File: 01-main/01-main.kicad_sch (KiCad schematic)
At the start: 96 parts, among them J1 USB_C_Receptacle_USB2.0, J10 front, J11 ToF_R, J12 ToF_RB, J13 ToF_L, J14 ToF_LB, J15 PWR_board_GND, J16 PWR_board_GND, J17 PWR_board_VIN, J18 PWR_board_VOUT, J19 XT60_LiPo, J2 Motor_RF, J20 UI_conn, J21 LOADCELL_R, J22 LOADCELL_L, J23 Conn_01x08, J3 Motor_RB, J4 Motor_LF, J5 Motor_LB, J6 OpenMV, J7 Conn_01x10, J8 Top, J9 Conn_01x10, SW1 SW_RST, SW2 SW_BOOT0, U1 STM32H723ZETx, U10 REG 6V, U11 NJU77551F, U12 NJU77551F, U2 CH340E, U4 REG 3V3, U6 REG 5V, U7 REG 6V, U8 REG 6V, U9 REG 6V, Y1 32.768kHz, Y2 24MHz

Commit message: がんばる
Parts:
- removed C10: 4.7uF, symbol Device:C
- removed C11, C12, C13, C14, C16, C20, C21, C4, C5, C6, C7, C8: 100nF, symbol Device:C
- removed C15, C19, C9: 1uF, symbol Device:C
- removed C17, C18: 2.2uF, symbol Device:C
- removed C22, C23: 1.5pF, symbol Device:C
- removed C24, C25: 33pF, symbol Device:C
- removed C26, C27, C33, C35, C37, C39: 0.1u, symbol Device:C
- removed C28, C30: 10u, symbol Device:C
- removed C29, C31: 22u, symbol Device:C
- removed C32, C34, C36, C38: 0.33u, symbol Device:C
- removed D1, D2: LED, symbol Device:LED
- removed FB1: FerriteBead, symbol Device:FerriteBead
- removed J1: USB_C_Receptacle_USB2.0, symbol Connector:USB_C_Receptacle_USB2.0
- removed J10: front, symbol Connector_Generic:Conn_01x10
- removed J11: ToF_R, symbol Connector_Generic:Conn_01x04
- removed J12: ToF_RB, symbol Connector_Generic:Conn_01x04
- removed J13: ToF_L, symbol Connector_Generic:Conn_01x04
- removed J14: ToF_LB, symbol Connector_Generic:Conn_01x04
- removed J15, J16: PWR_board_GND, symbol Connector_Generic:Conn_01x01
- removed J17: PWR_board_VIN, symbol Connector_Generic:Conn_01x01
- removed J18: PWR_board_VOUT, symbol Connector_Generic:Conn_01x01
- removed J19: XT60_LiPo, symbol Connector_Generic:Conn_01x02
- removed J2: Motor_RF, symbol Connector_Generic:Conn_01x03
- removed J20: UI_conn, symbol Connector_Generic:Conn_01x04
- removed J21: LOADCELL_R, symbol Connector_Generic:Conn_01x04
- removed J22: LOADCELL_L, symbol Connector_Generic:Conn_01x04
- removed J23: Conn_01x08, symbol Connector_Generic:Conn_01x08
- removed J3: Motor_RB, symbol Connector_Generic:Conn_01x03
- removed J6: OpenMV, symbol Connector_Generic:Conn_01x04
- removed J7, J9: Conn_01x10, symbol Connector_Generic:Conn_01x10
- removed J8: Top, symbol Connector_Generic:Conn_02x03_Counter_Clockwise
- removed R6: 330k, symbol Device:R
- removed R7, R8: 330, symbol Device:R
- removed SW1: SW_RST, symbol Switch:SW_Push
- removed SW2: SW_BOOT0, symbol Switch:SW_SPDT
- removed U1: STM32H723ZETx, Package_QFP:LQFP-144_20x20mm_P0.5mm, symbol MCU_ST_STM32H7:STM32H723ZETx
- removed U10, U7, U8, U9: REG 6V, Package_TO_SOT_SMD:TO-252-2, symbol Regulator_Linear:LF50_TO252
- removed U11, U12: NJU77551F, Package_TO_SOT_SMD:SOT-23-5, symbol Amplifier_Operational:OPA196xDBV
- removed U13: ~, symbol S11059:S11059
- removed U2: CH340E, Package_SO:MSOP-10_3x3mm_P0.5mm, symbol Interface_USB:CH340E
- removed U3: ~, symbol MPU6050:MPU6050
- removed U4: REG 3V3, Package_TO_SOT_SMD:TO-252-2, symbol Regulator_Linear:LF33_TO252
- removed U5: ~, symbol BNO055:AE-BNO055-BO
- removed U6: REG 5V, Package_TO_SOT_SMD:TO-252-2, symbol Regulator_Linear:LF50_TO252
- removed Y1: 32.768kHz, symbol Device:Crystal
- removed Y2: 24MHz, symbol Device:Crystal
- added J2: WRITER CONN, Connector_PinHeader_2.54mm:PinHeader_2x04_P2.54mm_Vertical, symbol Connector_Generic:Conn_02x04_Counter_Clockwise
- added J2: LOADCELL_R, symbol Connector_Generic:Conn_01x04
- added J3: LOADCELL_L, symbol Connector_Generic:Conn_01x04
- added J6, J7: Motor_R1, symbol Connector_Generic:Conn_01x03
- added J8: ToLINE, symbol Connector_Generic:Conn_01x04
- added Q1: 2SA1015, Package_TO_SOT_THT:TO-92_Inline, symbol Transistor_BJT:2SA1015
- added R14, R15, R16: 330k, symbol Device:R
- added U2: STM32F446RETx, Package_QFP:LQFP-64_10x10mm_P0.5mm, symbol MCU_ST_STM32F4:STM32F446RETx
- added U2: MAX485E, symbol Interface_UART:MAX485E
- added U3: ~, symbol BNO055:AE-BNO055-BO
- added U5, U6: NJU77551F, Package_TO_SOT_SMD:SOT-23-5, symbol Amplifier_Operational:OPA196xDBV
- C1: value 100nF -> 0.1u
- C2: value 100nF -> 100n
- C3: value 100nF -> 4.7u
- J4: value Motor_LF -> Motor_R1
- J5: value Motor_LB -> Motor_R1
- R1: value 10K -> 220
- R12, R9: value 330k -> 330
- R2: value 5.1k -> 7.5k
- R3: value 5.1k -> 2.2k
- R4: value R -> 2.2k
- R5: value R -> 10k; footprint (none) -> Resistor_SMD:R_0805_2012Metric; LCSC (none) -> C17414
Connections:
- net MotorLB is gone; now on net GND: J5.3 (Pin_3)
- net MotorLF is gone; now on net GND: J4.3 (Pin_3)
- net +3V3: now also J2.4 (Pin_4), J2.8 (Pin_8), J3.4 (Pin_4), U2.1 (VBAT), U2.13 (VDDA), U2.19 (VDD), U2.32 (VDD), U2.48 (VDD), U2.64 (VDD), U3.1 (VIN), U5.5 (V+), U6.5 (V+); no longer C1.1, C2.1, C3.1
- net +5V: now also C1.1, R3.1, Q1.2 (C), U2.8 (VCC)
- net BOOT0: now also R5.1, J2.5 (Pin_5), U2.60 (BOOT0); no longer R1.2
- net GND: now also C2.1, R1.2, R4.1, R5.2, J2.1 (Pin_1), J2.6 (Pin_6), J3.1 (Pin_1), J6.3 (Pin_3), J7.3 (Pin_3), R15.2, U2.12 (VSSA), U2.18 (VSS), U2.31 (VSS), U2.47 (VSS), U2.5 (GND), U2.63 (VSS), U3.2 (GND), U5.2 (V-), U6.2 (V-); no longer C2.2, J4.2 (Pin_2), J5.2 (Pin_2), R2.2, R3.2, R4.2
- net I2C1_SCL: now also U2.58 (PB6), U3.4 (SCL)
- net I2C1_SDA: now also U2.59 (PB7), U3.3 (SDA)
- net I2C2_SCL: now also U2.29 (PB10)
- net I2C2_SDA: now also U2.53 (PC12)
- net LOADCEL_L: now also R16.1, U6.1; no longer R12.1
- net LOADCEL_R: now also R14.1, U5.1; no longer R9.1
- net NRST: now also C2.2, J2.3 (Pin_3), U2.7 (NRST)
- net UART1_RX: now also J2.2 (Pin_2), U2.43 (PA10)
- net UART1_TX: now also J2.4 (Pin_4), U2.42 (PA9)
- net at R10.1: now also R14.2, U5.4 (-)
- net at R11.2: now also R15.1, U6.3 (+)
- net at R13.1: now also R9.2, U5.3 (+); no longer R10.2
- net at R11.1: now also J3.2 (Pin_2); no longer R12.2
- net STS_SIG: now reaches J4.1 (Pin_1)
- net STS_SIG: now also J5.1 (Pin_1), J6.1 (Pin_1), J7.1 (Pin_1), U2.6 (A)
- net at R2.1: now also Q1.3 (B)
- net at R1.1: now also Q1.1 (E), U2.2 (~{RE}), U2.3 (DE)
- net Buzzer: no longer names the net of BZ1.1 (-)
- new net: J3.3 (Pin_3), R12.2
- new net: R12.1, R16.2, U6.4 (-)
- new net: J2.2 (Pin_2), R9.1
- new net: J2.3 (Pin_3), R10.2
- new net: C3.1, U2.30 (VCAP_1)
- new net: R3.2, R4.2, U2.7 (B)
- new net: R2.2, U2.4 (DI)
- new net +6V: J4.2 (Pin_2), J5.2 (Pin_2), J6.2 (Pin_2), J7.2 (Pin_2)
- no-connect marks 73 -> 6
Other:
- note removed: "CONN"
- note removed: "LINE SENSOR"
- note removed: "LOADCELL"
- note removed: "MOTOR"
- note removed: "POWER"
- note removed: "SENSOR"
- note removed: "STM32H723ZGT6"

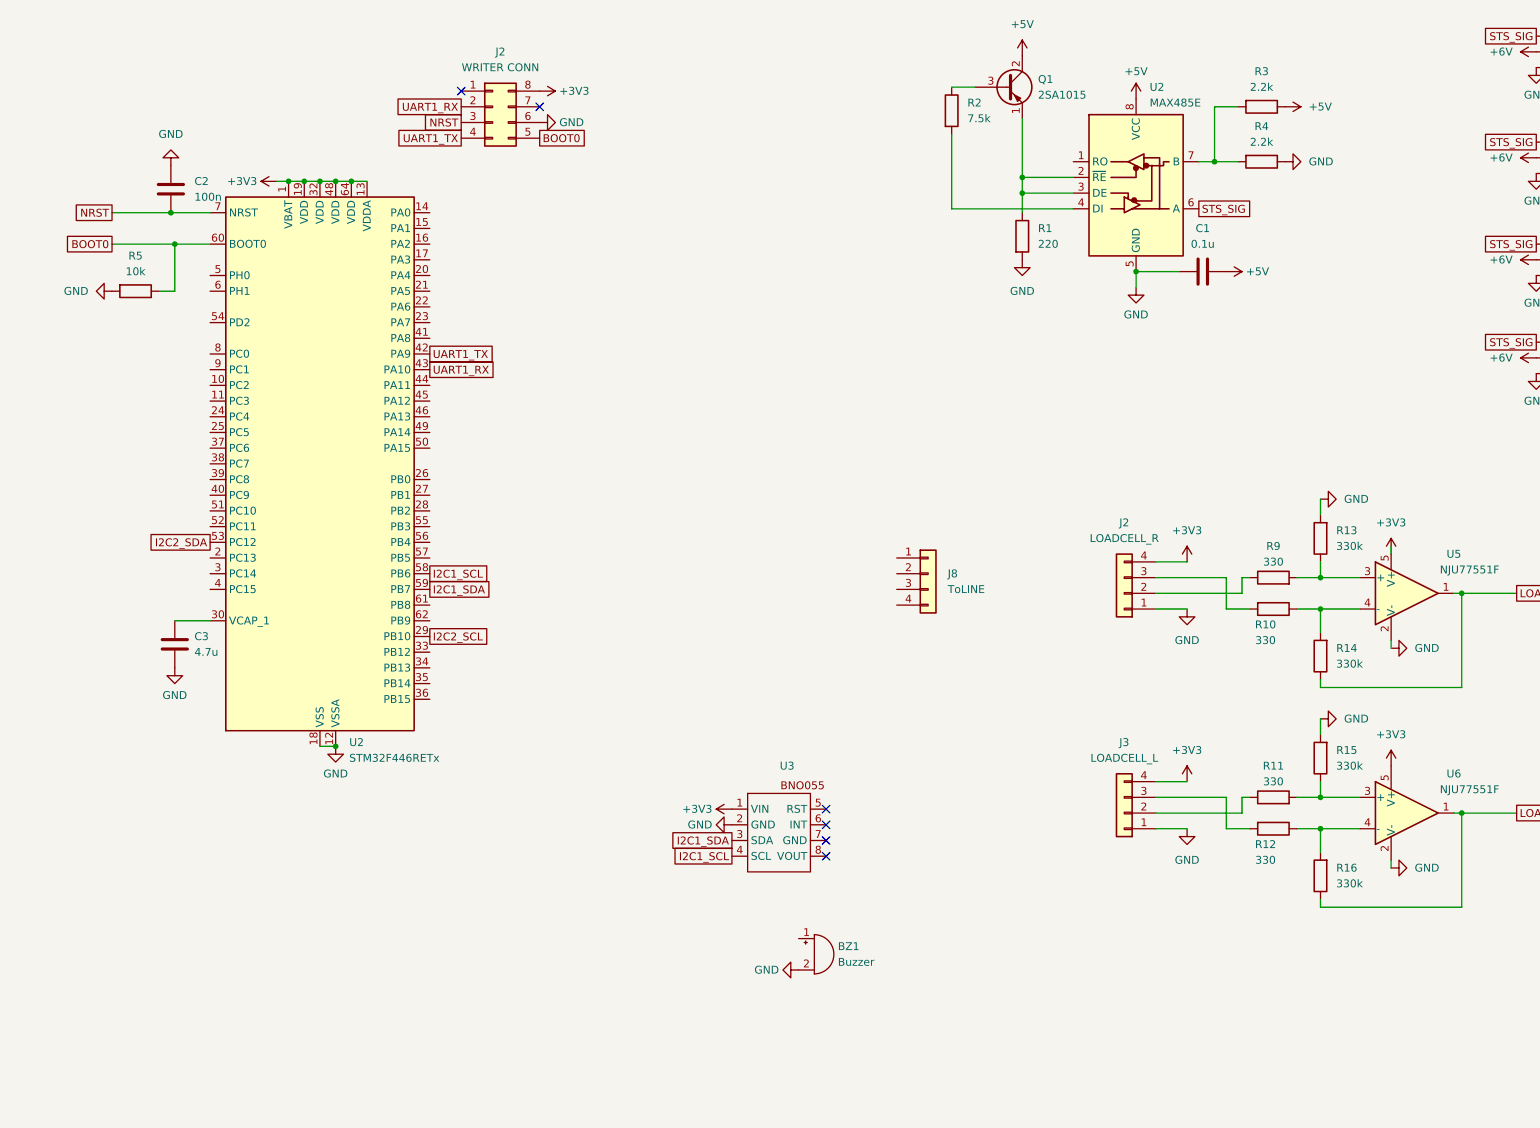
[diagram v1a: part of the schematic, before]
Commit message: いっぱい増えた
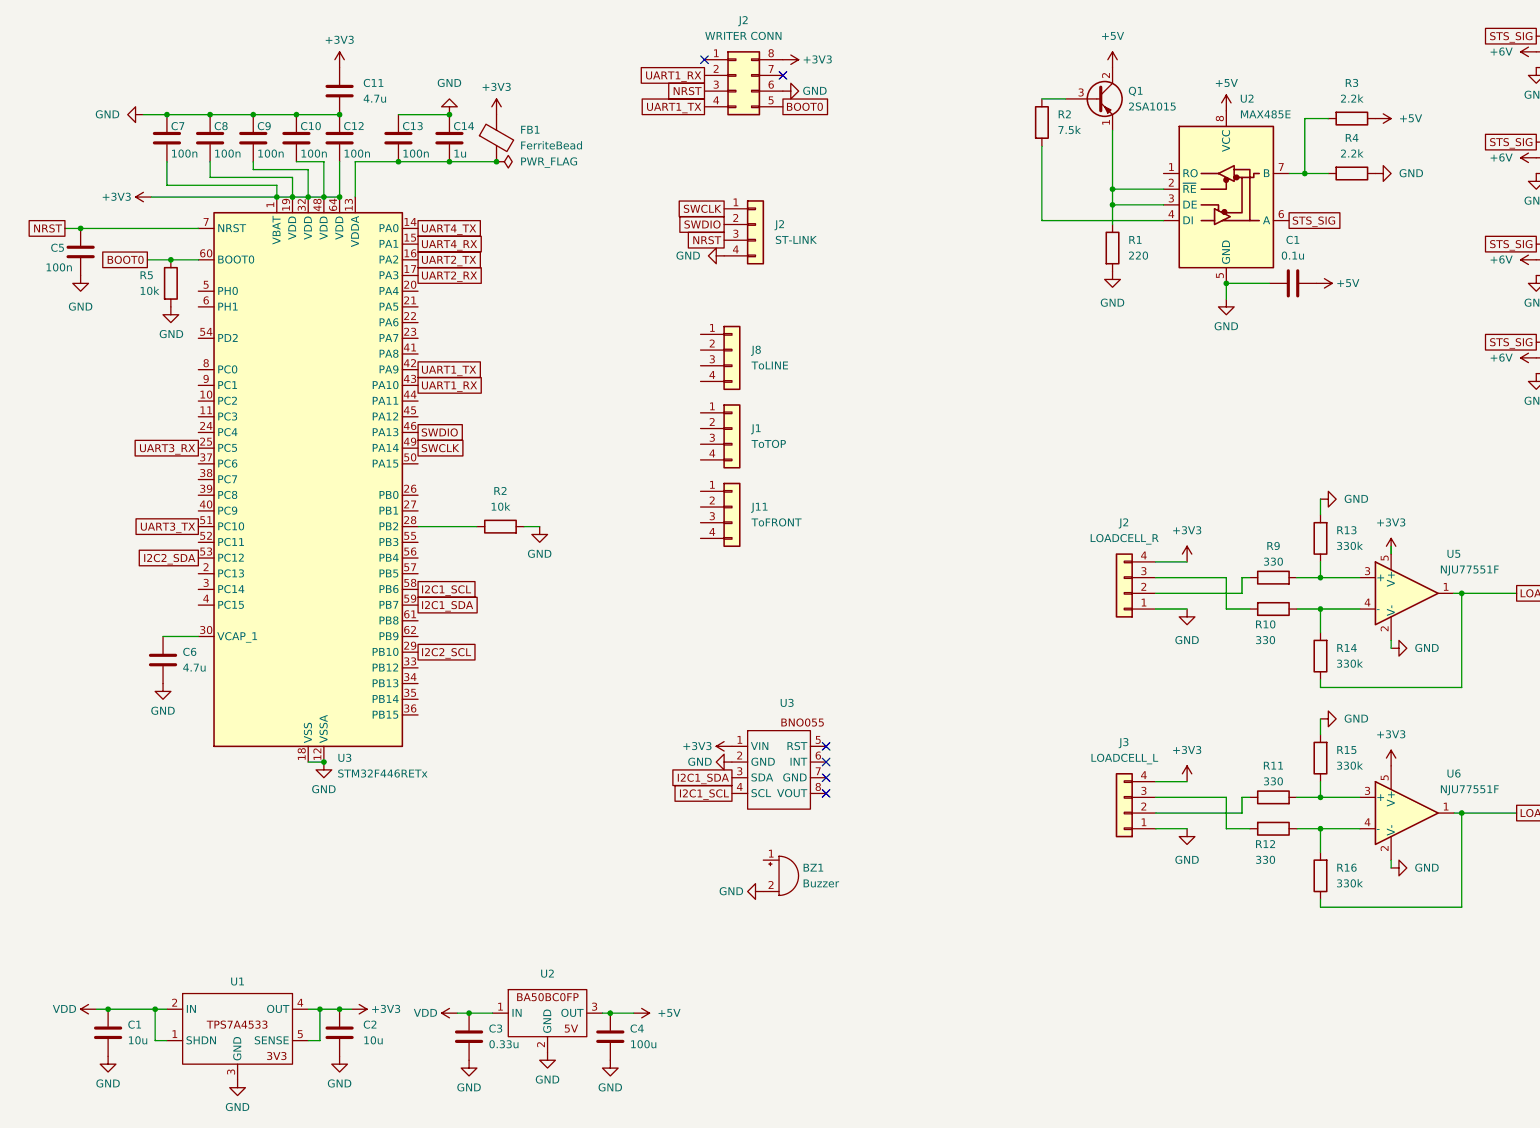
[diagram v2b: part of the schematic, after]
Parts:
- removed U2: STM32F446RETx, Package_QFP:LQFP-64_10x10mm_P0.5mm, symbol MCU_ST_STM32F4:STM32F446RETx
- added C1: 10u, Capacitor_SMD:C_0603_1608Metric, symbol Device:C
- added C10, C12, C13, C5, C7, C8, C9: 100n, Capacitor_SMD:C_0402_1005Metric, symbol Device:C
- added C11, C6: 4.7u, Capacitor_SMD:C_0402_1005Metric, symbol Device:C
- added C14: 1u, Capacitor_SMD:C_0402_1005Metric, symbol Device:C
- added C4: 100u, Capacitor_SMD:C_1206_3216Metric, symbol Device:C
- added FB1: FerriteBead, Resistor_SMD:R_0805_2012Metric, symbol Device:FerriteBead
- added J1: ToTOP, symbol Connector_Generic:Conn_01x04
- added J11: ToFRONT, symbol Connector_Generic:Conn_01x04
- added J2: ST-LINK, Connector_PinHeader_2.54mm:PinHeader_1x04_P2.54mm_Vertical, symbol Connector_Generic:Conn_01x04
- added R2: 10k, Resistor_SMD:R_0603_1608Metric, symbol Device:R
- added U1: ~, Package_TO_SOT_SMD:SOT-223-6, symbol JLCPCB_items:TPS7A4533DCQR
- added U2: ~, Package_TO_SOT_SMD:TO-252-3_TabPin2, symbol JLCPCB_items:BA50BC0FP
- added U3: STM32F446RETx, Package_QFP:LQFP-64_10x10mm_P0.5mm, symbol MCU_ST_STM32F4:STM32F446RETx
- C2: value 100n -> 10u; footprint (none) -> Capacitor_SMD:C_0603_1608Metric; LCSC (none) -> C3015157
- C3: value 4.7u -> 0.33u; footprint (none) -> Capacitor_SMD:C_0805_2012Metric; LCSC (none) -> C2961026
- R5: footprint Resistor_SMD:R_0805_2012Metric -> Resistor_SMD:R_0603_1608Metric; LCSC C17414 -> C137819
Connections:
- net +3V3: now also C2.1, C10.2, C11.1, C12.2, C7.2, C8.2, C9.2, FB1.1, U1.4 (OUT), U1.5 (SENSE), U3.1 (VBAT), U3.19 (VDD), U3.32 (VDD), U3.48 (VDD), U3.64 (VDD)
- net +5V: now also C4.1, U2.3 (OUT)
- net BOOT0: now also U3.60 (BOOT0)
- net GND: now also C2.2, C1.2, C10.1, C11.2, C12.1, C13.1, C14.1, C4.2, C5.1, C6.2, C7.1, C8.1, C9.1, J2.4 (Pin_4), R2.2, U1.3 (GND), U1.6 (GND), U2.2 (GND), U3.12 (VSSA), U3.18 (VSS), U3.31 (VSS), U3.47 (VSS), U3.63 (VSS); no longer C2.1
- net I2C1_SCL: now also U3.58 (PB6)
- net I2C1_SDA: now also U3.59 (PB7)
- net I2C2_SCL: now also U3.29 (PB10)
- net I2C2_SDA: now also U3.53 (PC12)
- net NRST: now also C5.2, J2.3 (Pin_3), U3.7 (NRST); no longer C2.2
- net UART1_RX: now also U3.43 (PA10)
- net UART1_TX: now also U3.42 (PA9)
- net VDD: now reaches C3.1
- net VDD: now also C1.1, U1.1 (SHDN), U1.2 (IN), U2.1 (IN)
- new net: C13.2, C14.2, FB1.2, U3.13 (VDDA)
- new net: R2.1, U3.28 (PB2)
- new net: C6.1, U3.30 (VCAP_1)
- new net SWCLK: J2.1 (Pin_1), U3.49 (PA14)
- new net SWDIO: J2.2 (Pin_2), U3.46 (PA13)
- new net UART2_RX: U3.17 (PA3)
- new net UART2_TX: U3.16 (PA2)
- new net UART3_RX: U3.25 (PC5)
- new net UART3_TX: U3.51 (PC10)
- new net UART4_RX: U3.15 (PA1)
- new net UART4_TX: U3.14 (PA0)
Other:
- moved on the sheet: BZ1, C1, J8, Q1, R1, R2, R3, R4, U2, U3
